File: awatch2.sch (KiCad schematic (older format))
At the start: 15 parts

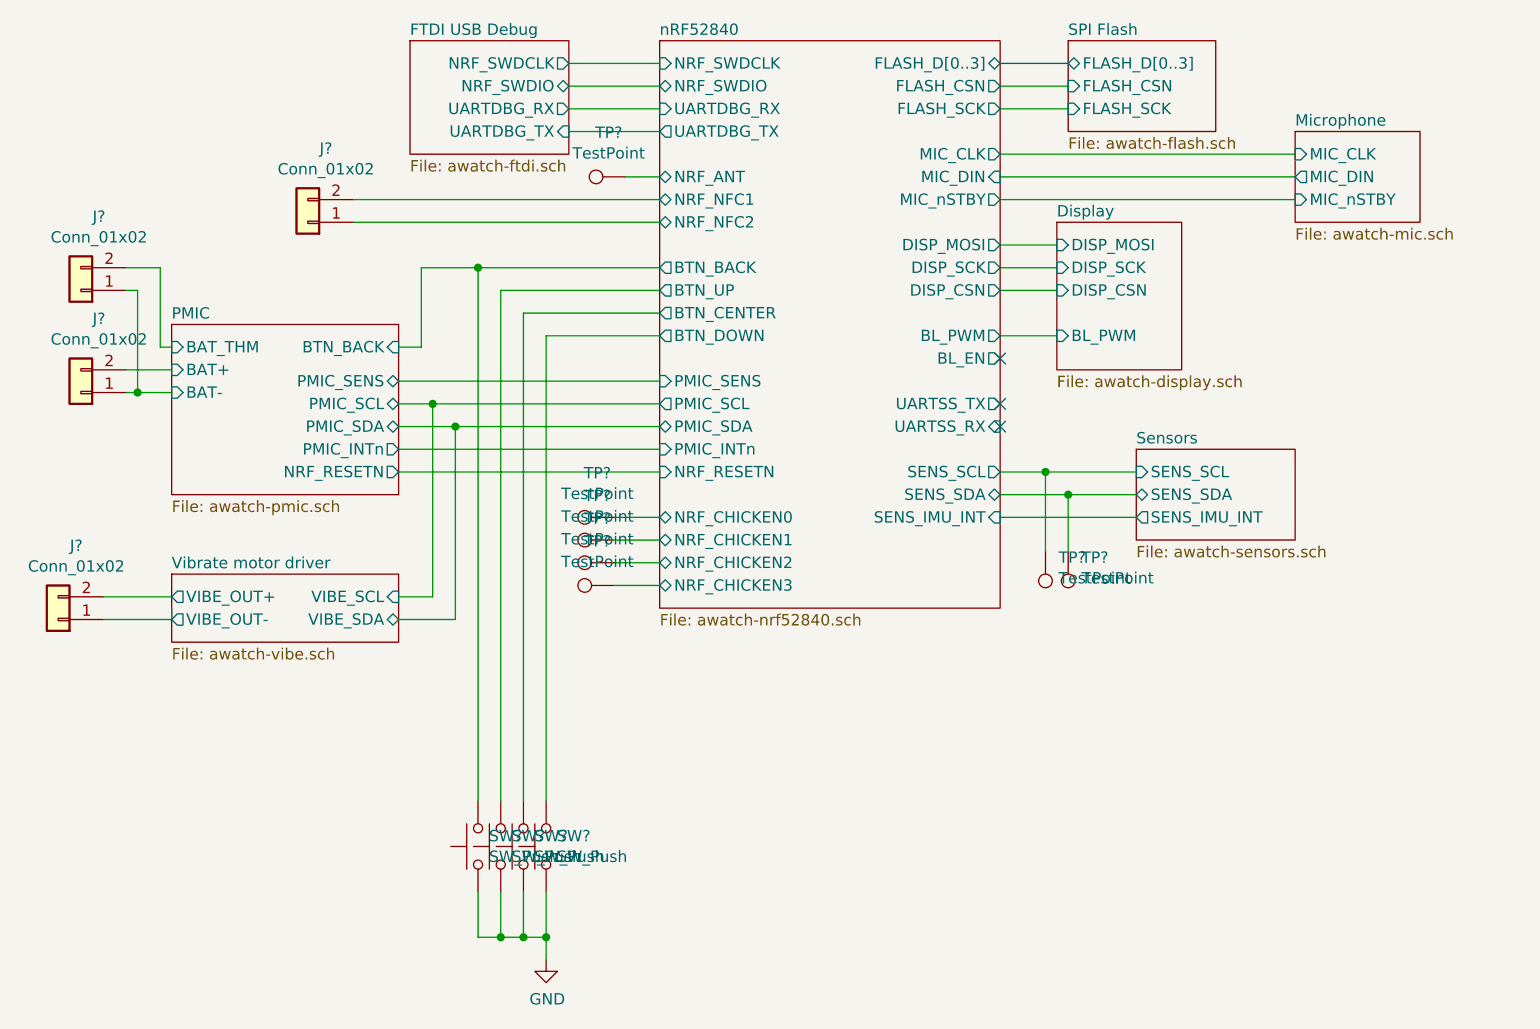
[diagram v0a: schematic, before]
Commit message: annotate all
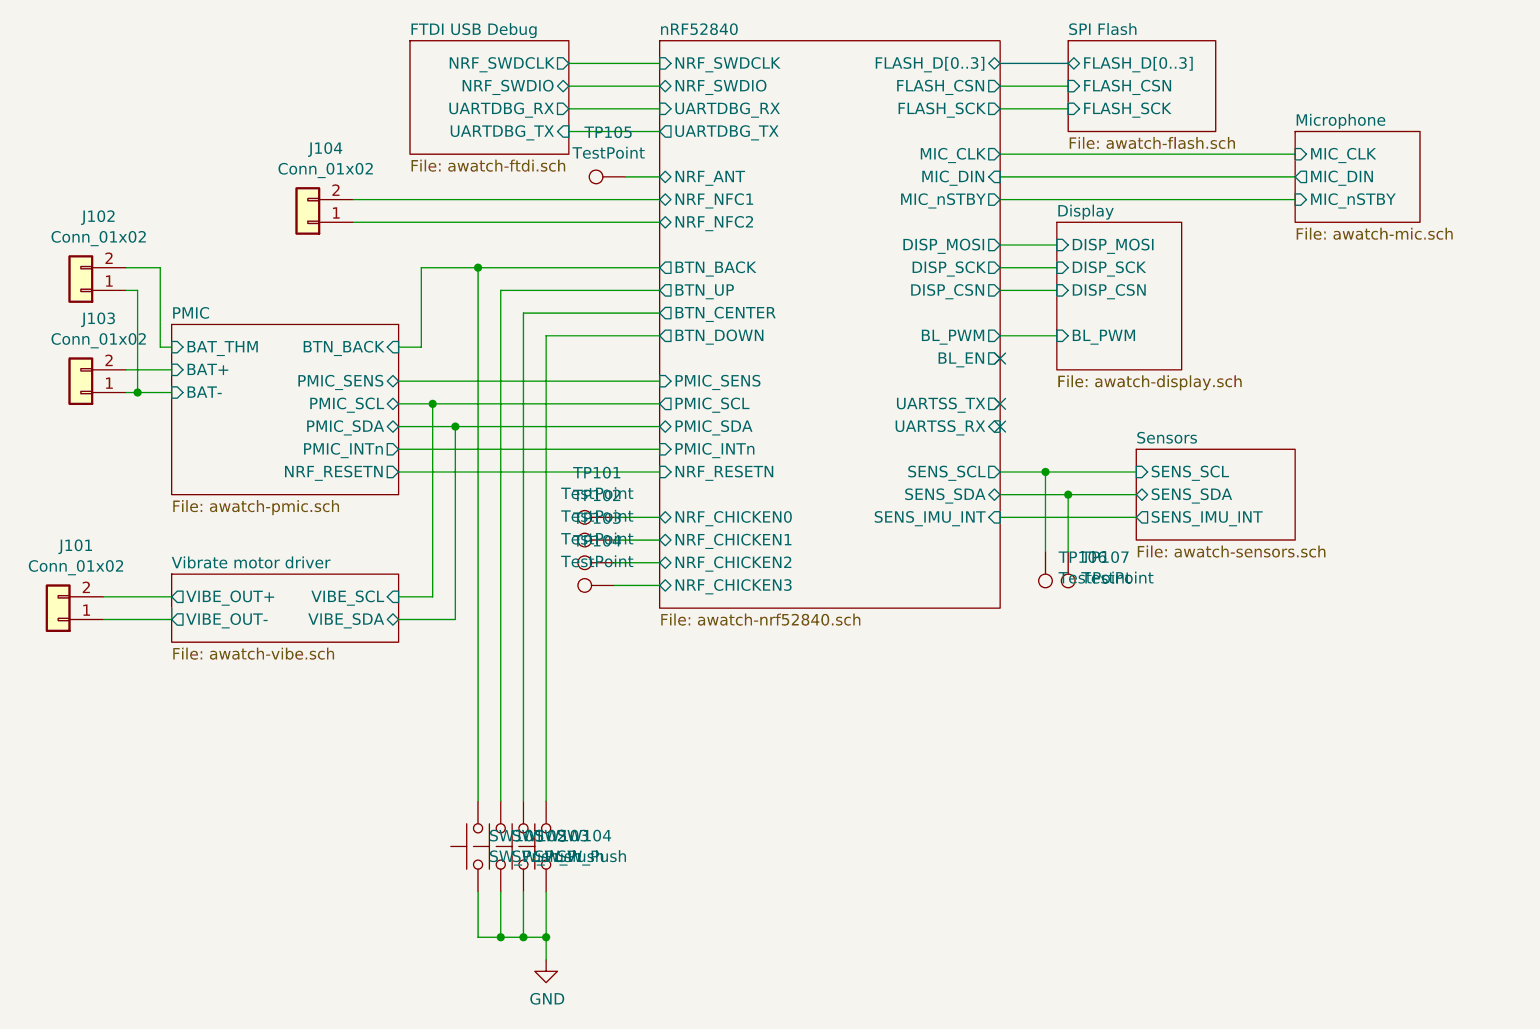
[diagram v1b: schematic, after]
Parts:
- gave numbers to parts that had none: 15
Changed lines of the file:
@@
 	5150 2250 4750 2250
 $Comp
-L Connector:TestPoint TP?
+L Connector:TestPoint TP101
 U 1 1 5C7B2BD0
 P 4950 3950
-F 0 "TP?" V 5145 4024 50  0000 C CNN
+F 0 "TP101" V 5145 4024 50  0000 C CNN
 F 1 "TestPoint" V 5054 4024 50  0000 C CNN
 F 2 "" H 5150 3950 50  0001 C CNN
@@
 	4950 3950 5150 3950
 $Comp
-L Connector:TestPoint TP?
+L Connector:TestPoint TP102
 U 1 1 5C7B30D8
 P 4950 4050
-F 0 "TP?" V 5145 4124 50  0000 C CNN
+F 0 "TP102" V 5145 4124 50  0000 C CNN
 F 1 "TestPoint" V 5054 4124 50  0000 C CNN
 F 2 "" H 5150 4050 50  0001 C CNN
@@
 	4950 4050 5150 4050
 $Comp
-L Connector:TestPoint TP?
+L Connector:TestPoint TP103
 U 1 1 5C7B35EE
 P 4950 4150
-F 0 "TP?" V 5145 4224 50  0000 C CNN
+F 0 "TP103" V 5145 4224 50  0000 C CNN
 F 1 "TestPoint" V 5054 4224 50  0000 C CNN
 F 2 "" H 5150 4150 50  0001 C CNN
@@
 	4950 4150 5150 4150
 $Comp
-L Connector:TestPoint TP?
+L Connector:TestPoint TP104
 U 1 1 5C7B3B74
 P 4950 4250
-F 0 "TP?" V 5145 4324 50  0000 C CNN
+F 0 "TP104" V 5145 4324 50  0000 C CNN
 F 1 "TestPoint" V 5054 4324 50  0000 C CNN
 F 2 "" H 5150 4250 50  0001 C CNN
@@
 	4950 4250 5150 4250
 $Comp
-L Connector:TestPoint TP?
+L Connector:TestPoint TP105
 U 1 1 5C7B41B6
 P 5000 2450
-F 0 "TP?" V 5195 2524 50  0000 C CNN
+F 0 "TP105" V 5195 2524 50  0000 C CNN
 F 1 "TestPoint" V 5104 2524 50  0000 C CNN
 F 2 "" H 5200 2450 50  0001 C CNN
@@
 P 3600 2650
 AR Path="/5C357822/5C7B5026" Ref="J?"  Part="1"
-AR Path="/5C7B5026" Ref="J?"  Part="1"
-F 0 "J?" H 3520 2325 50  0000 C CNN
+AR Path="/5C7B5026" Ref="J104"  Part="1"
+F 0 "J104" H 3520 2325 50  0000 C CNN
 F 1 "Conn_01x02" H 3520 2416 50  0000 C CNN
 F 2 "" H 3600 2650 50  0001 C CNN
@@
 P 2600 2950
 AR Path="/5C357822/5C7B934C" Ref="J?"  Part="1"
-AR Path="/5C7B934C" Ref="J?"  Part="1"
-F 0 "J?" H 2520 2625 50  0000 C CNN
+AR Path="/5C7B934C" Ref="J102"  Part="1"
+F 0 "J102" H 2520 2625 50  0000 C CNN
 F 1 "Conn_01x02" H 2520 2716 50  0000 C CNN
 F 2 "" H 2600 2950 50  0001 C CNN
@@
 P 2600 3400
 AR Path="/5C357822/5C7BAE8F" Ref="J?"  Part="1"
-AR Path="/5C7BAE8F" Ref="J?"  Part="1"
-F 0 "J?" H 2520 3075 50  0000 C CNN
+AR Path="/5C7BAE8F" Ref="J103"  Part="1"
+F 0 "J103" H 2520 3075 50  0000 C CNN
 F 1 "Conn_01x02" H 2520 3166 50  0000 C CNN
 F 2 "" H 2600 3400 50  0001 C CNN
@@
 	4550 5800 4450 5800
 $Comp
-L power:GND #PWR?
+L power:GND #PWR0119
 U 1 1 5C7C612C
 P 4650 5900
-F 0 "#PWR?" H 4650 5650 50  0001 C CNN
+F 0 "#PWR0119" H 4650 5650 50  0001 C CNN
 F 1 "GND" H 4655 5727 50  0000 C CNN
 F 2 "" H 4650 5900 50  0001 C CNN
@@
 Connection ~ 4650 5800
 $Comp
-L Switch:SW_Push SW?
+L Switch:SW_Push SW101
 U 1 1 5C7C7C50
 P 4350 5400
-F 0 "SW?" V 4396 5352 50  0000 R CNN
+F 0 "SW101" V 4396 5352 50  0000 R CNN
 F 1 "SW_Push" V 4305 5352 50  0000 R CNN
 F 2 "" H 4350 5600 50  0001 C CNN
@@
 $EndComp
 $Comp
-L Switch:SW_Push SW?
+L Switch:SW_Push SW102
 U 1 1 5C7CB63F
 P 4450 5400
-F 0 "SW?" V 4496 5352 50  0000 R CNN
+F 0 "SW102" V 4496 5352 50  0000 R CNN
 F 1 "SW_Push" V 4405 5352 50  0000 R CNN
 F 2 "" H 4450 5600 50  0001 C CNN
@@
 $EndComp
 $Comp
-L Switch:SW_Push SW?
+L Switch:SW_Push SW103
 U 1 1 5C7CB661
 P 4550 5400
-F 0 "SW?" V 4596 5352 50  0000 R CNN
+F 0 "SW103" V 4596 5352 50  0000 R CNN
 F 1 "SW_Push" V 4505 5352 50  0000 R CNN
 F 2 "" H 4550 5600 50  0001 C CNN
@@
 $EndComp
 $Comp
-L Switch:SW_Push SW?
+L Switch:SW_Push SW104
 U 1 1 5C7CB685
 P 4650 5400
-F 0 "SW?" V 4696 5352 50  0000 R CNN
+F 0 "SW104" V 4696 5352 50  0000 R CNN
 F 1 "SW_Push" V 4605 5352 50  0000 R CNN
 F 2 "" H 4650 5600 50  0001 C CNN
@@
 	6650 3950 7250 3950
 $Comp
-L Connector:TestPoint TP?
+L Connector:TestPoint TP106
 U 1 1 5C7D0B25
 P 6850 4100
-F 0 "TP?" H 6792 4127 50  0000 R CNN
+F 0 "TP106" H 6792 4127 50  0000 R CNN
 F 1 "TestPoint" H 6792 4218 50  0000 R CNN
 F 2 "" H 7050 4100 50  0001 C CNN
@@
 	6850 3750 7250 3750
 $Comp
-L Connector:TestPoint TP?
+L Connector:TestPoint TP107
 U 1 1 5C7D1D36
 P 6950 4100
-F 0 "TP?" H 6892 4127 50  0000 R CNN
+F 0 "TP107" H 6892 4127 50  0000 R CNN
 F 1 "TestPoint" H 6892 4218 50  0000 R CNN
 F 2 "" H 7150 4100 50  0001 C CNN
@@
 P 2500 4400
 AR Path="/5C357822/5C7D74BF" Ref="J?"  Part="1"
-AR Path="/5C7D74BF" Ref="J?"  Part="1"
-F 0 "J?" H 2420 4075 50  0000 C CNN
+AR Path="/5C7D74BF" Ref="J101"  Part="1"
+F 0 "J101" H 2420 4075 50  0000 C CNN
 F 1 "Conn_01x02" H 2420 4166 50  0000 C CNN
 F 2 "" H 2500 4400 50  0001 C CNN
